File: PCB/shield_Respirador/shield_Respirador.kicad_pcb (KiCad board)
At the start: 2 copper layers, 137.3 x 102 mm, 29 parts, among them P1 Digital, P10 CONN_01X01, P11 CONN_01X01, P12 CONN_01X01, P13 CONN_01X01, P2 Power, P3 Analog, P4 Analog, P5 PWM, P6 PWM, P7 Communication, P8 CONN_01X01, P9 CONN_01X01

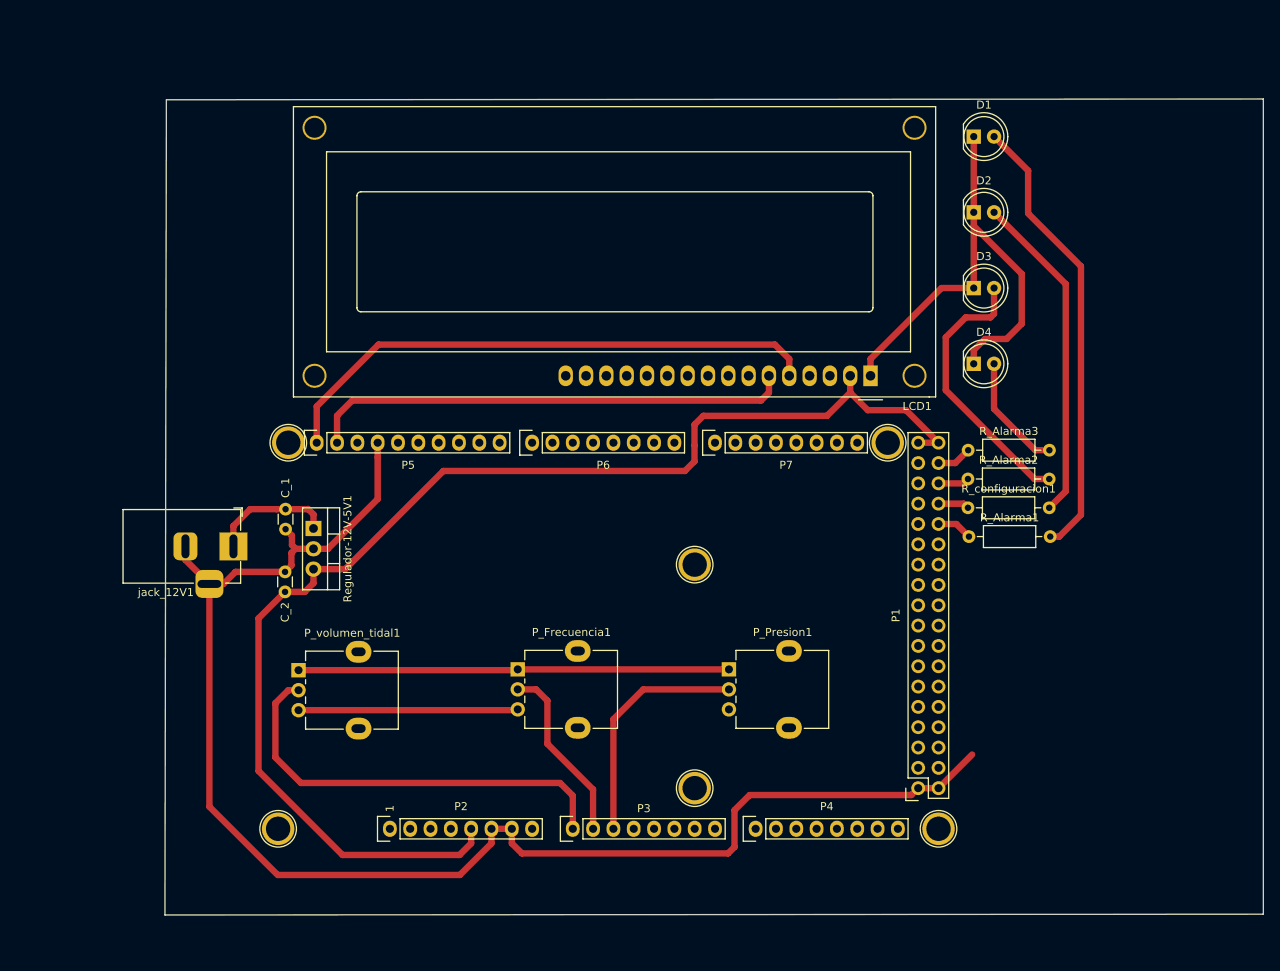
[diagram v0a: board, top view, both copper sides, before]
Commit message: version 0.4
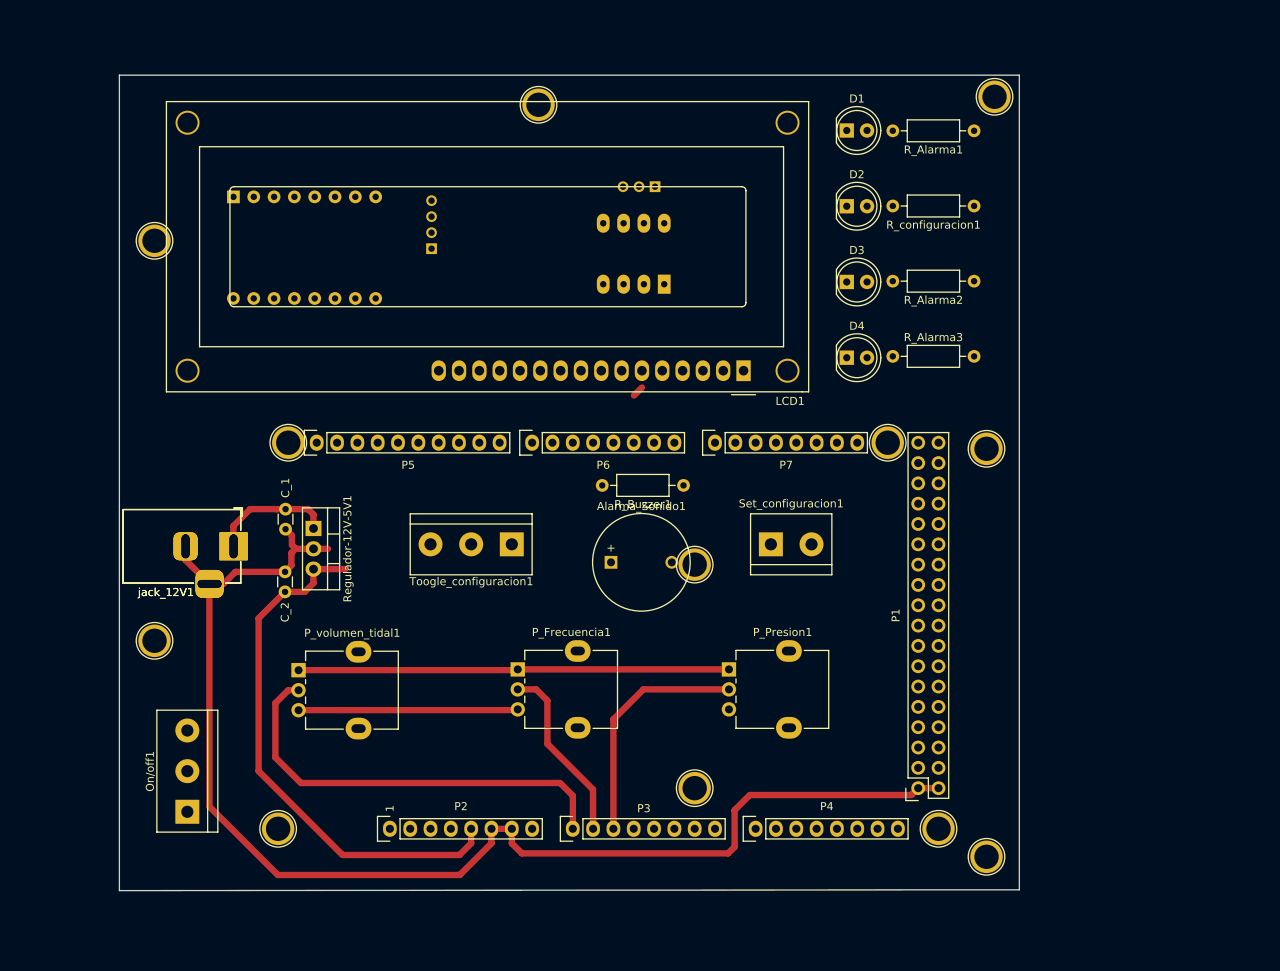
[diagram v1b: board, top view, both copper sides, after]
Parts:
- added Alarma_Sonido1: Buzzer, Buzzer_Beeper:MagneticBuzzer_ProSignal_ABI-009-RC, F.Cu at (159.0, 85.8)
- added Drivermotor1: Pololu_Breakout_DRV8825, Module:Pololu_Breakout-16_15.2x20.3mm, B.Cu at (111.8, 40.1)
- added Final_De_Carrera1: Conn_01x03_Female, Connector_PinSocket_2.00mm:PinSocket_1x03_P2.00mm_Vertical, B.Cu at (164.5, 38.9)
- added On/off1: SW_DPDT_x2, TerminalBlock:TerminalBlock_bornier-3_P5.08mm, F.Cu at (106.0, 117.0)
- added P10: CONN_01X01, Socket_Arduino_Mega:Arduino_1pin, F.Cu at (101.9, 95.6)
- added P10: CONN_01X01, Socket_Arduino_Mega:Arduino_1pin, F.Cu at (149.9, 28.6)
- added P10: CONN_01X01, Socket_Arduino_Mega:Arduino_1pin, F.Cu at (101.9, 45.6)
- added P10: CONN_01X01, Socket_Arduino_Mega:Arduino_1pin, F.Cu at (205.9, 71.6)
- added P10: CONN_01X01, Socket_Arduino_Mega:Arduino_1pin, F.Cu at (206.9, 27.6)
- added P10: CONN_01X01, Socket_Arduino_Mega:Arduino_1pin, F.Cu at (205.9, 122.6)
- added R_Buzzer1: 220, Resistor_THT:R_Axial_DIN0207_L6.3mm_D2.5mm_P10.16mm_Horizontal, F.Cu at (168.0, 76.2)
- added Sensor_Presion1: MPXA6115A, Package_DIP:DIP-8_W7.62mm_LongPads, B.Cu at (165.6, 51.1)
- added Set_configuracion1: SW_Push, TerminalBlock:TerminalBlock_bornier-2_P5.08mm, F.Cu at (178.9, 83.6)
- added Toogle_configuracion1: SW_Push_SPDT, TerminalBlock:TerminalBlock_bornier-3_P5.08mm, F.Cu at (146.6, 83.6)
- added conector_motor1: Conn_01x04_Female, Connector_PinSocket_2.00mm:PinSocket_1x04_P2.00mm_Vertical, B.Cu at (136.5, 46.6)
- added jack_12V1: Alimentacion_12V, Connector_BarrelJack:BarrelJack_Horizontal, F.Cu at (111.8, 83.8)
- moved R_Alarma1 50.7 mm to (204.3, 31.9), turned to 180 degrees
- moved R_configuracion1 37.7 mm to (204.3, 41.3), turned to 180 degrees
- moved R_Alarma2 24.7 mm to (204.3, 50.7), turned to 180 degrees
- moved D1 15.9 mm to (188.4, 31.8)
- moved D2 15.9 mm to (188.4, 41.3)
- moved D3 15.9 mm to (188.4, 50.8)
- moved D4 15.9 mm to (188.4, 60.2)
- moved LCD1 15.9 mm to (175.5, 61.9)
- moved R_Alarma3 15.0 mm to (194.2, 60.1)
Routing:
- net +5V: track 160.1 -> 66.8 mm
- net GND: track 244.0 -> 160.8 mm
- net /SCL: track 69.7 -> 0.00 mm
- net /SDA: track 60.7 -> 1.41 mm
- net Net-(D1-Pad2): track 56.8 -> 0.00 mm
- net Net-(D2-Pad2): track 41.5 -> 0.00 mm
- net Net-(D3-Pad2): track 34.6 -> 0.00 mm
- net Net-(D4-Pad2): track 14.7 -> 0.00 mm
- net /29: track 4.45 -> 0.00 mm
- net /23: track 4.37 -> 0.00 mm
- net /25: track 3.90 -> 0.00 mm
- net /27: track 3.89 -> 0.00 mm
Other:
- board size 137.3 x 102 mm -> 112.5 x 101.9 mm

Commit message: version 0.5 se termina esquematico y renderizacion
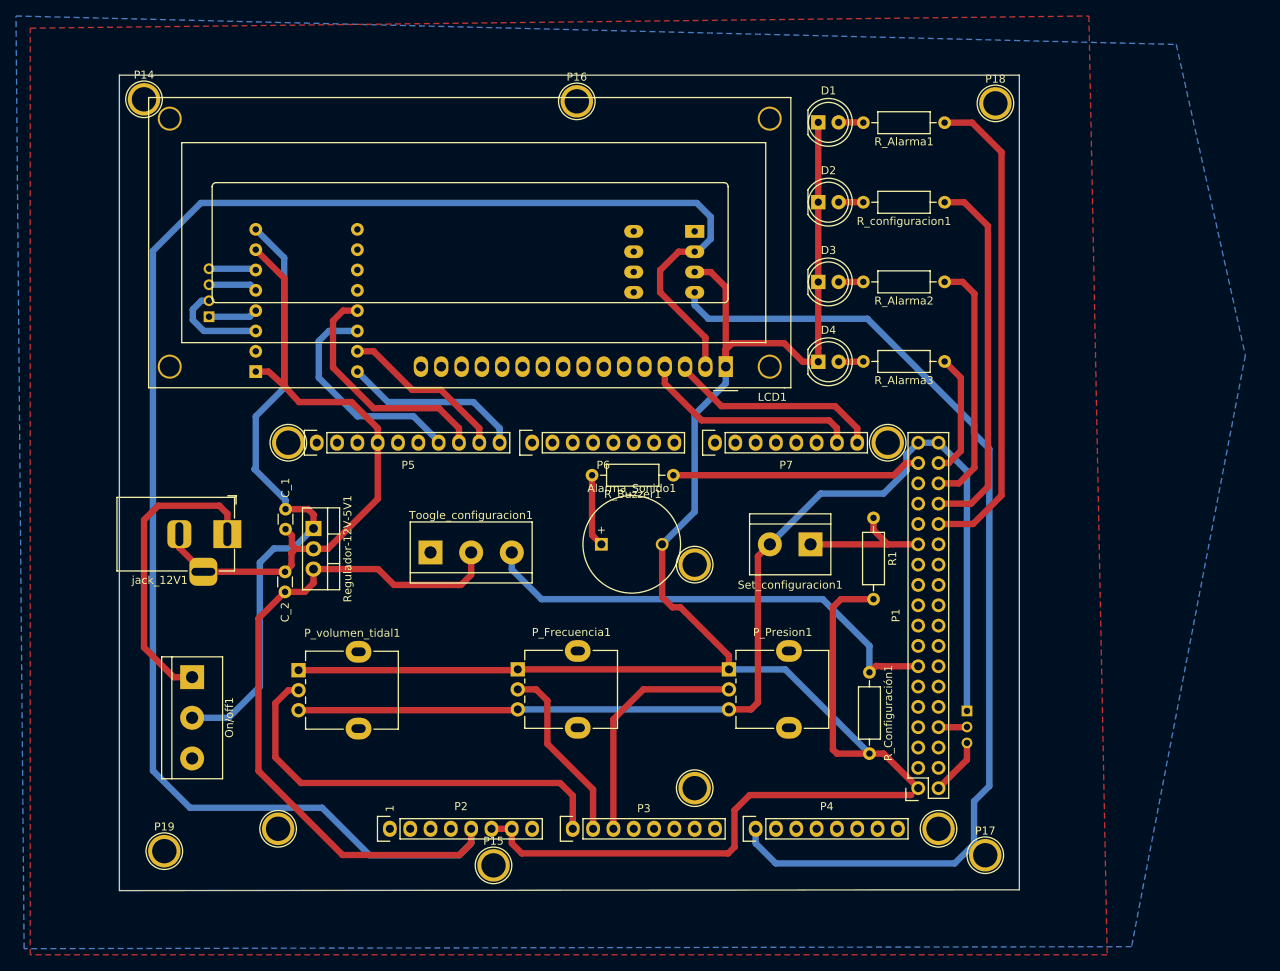
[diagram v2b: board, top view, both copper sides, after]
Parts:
- removed the P10 at (101.9, 95.6)
- removed the P10 at (149.9, 28.6)
- removed the P10 at (101.9, 45.6)
- removed the P10 at (205.9, 71.6)
- removed the P10 at (206.9, 27.6)
- removed the P10 at (205.9, 122.6)
- removed the jack_12V1 at (111.8, 83.8) (x2)
- added P14: CONN_01X01, Socket_Arduino_Mega:Arduino_1pin, F.Cu at (100.6, 27.9)
- added P15: CONN_01X01, Socket_Arduino_Mega:Arduino_1pin, F.Cu at (144.3, 123.7)
- added P16: CONN_01X01, Socket_Arduino_Mega:Arduino_1pin, F.Cu at (154.7, 28.2)
- added P17: CONN_01X01, Socket_Arduino_Mega:Arduino_1pin, F.Cu at (205.7, 122.4)
- added P18: CONN_01X01, Socket_Arduino_Mega:Arduino_1pin, F.Cu at (207.0, 28.4)
- added P19: CONN_01X01, Socket_Arduino_Mega:Arduino_1pin, F.Cu at (103.1, 121.9)
- added R1: R, Resistor_THT:R_Axial_DIN0207_L6.3mm_D2.5mm_P10.16mm_Horizontal, F.Cu at (191.8, 80.3)
- added R_Configuración1: 220, Resistor_THT:R_Axial_DIN0207_L6.3mm_D2.5mm_P10.16mm_Horizontal, F.Cu at (191.3, 99.6)
- added jack_12V1: Alimentacion_12V, Connector_BarrelJack:BarrelJack_Horizontal, F.Cu at (111.0, 82.3)
- Drivermotor1: value Pololu_Breakout_DRV8825 -> DRV8825
- moved Final_De_Carrera1 76.3 mm to (203.5, 104.4), turned to 180 degrees
- moved conector_motor1 29.1 mm to (108.7, 55.1)
- moved Drivermotor1 22.0 mm to (114.6, 62.0), turned to 0 degrees
- moved On/off1 16.8 mm to (106.6, 100.2), turned to 270 degrees
- moved Toogle_configuracion1 10.2 mm to (136.4, 84.6), turned to 0 degrees
- moved Sensor_Presion1 7.62 mm to (169.4, 44.5), turned to 180 degrees
- moved R_Alarma3 6.51 mm to (200.7, 60.7), turned to 180 degrees
- moved Set_configuracion1 4.95 mm to (183.9, 83.6), turned to 180 degrees
- moved R_Alarma1 3.82 mm to (200.7, 30.9)
- moved R_configuracion1 3.71 mm to (200.7, 40.8)
- moved D1 3.70 mm to (184.9, 30.8)
- moved R_Alarma2 3.68 mm to (200.7, 50.8)
- moved D4 3.59 mm to (184.9, 60.7)
- moved D2 3.59 mm to (184.9, 40.8)
- moved D3 3.56 mm to (184.9, 50.8)
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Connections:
- Drivermotor1 pad 1: Net-(Drivermotor1-Pad1) -> GND
- Drivermotor1 pad 13: Net-(Drivermotor1-Pad13) -> /10(**)
- Drivermotor1 pad 14: Net-(Drivermotor1-Pad14) -> /11(**)
- Drivermotor1 pad 15: Net-(Drivermotor1-Pad15) -> /9(**)
- Drivermotor1 pad 16: Net-(Drivermotor1-Pad16) -> /8(**)
- Drivermotor1 pad 7: Net-(Drivermotor1-Pad7) -> GND
- Drivermotor1 pad 8: Net-(Drivermotor1-Pad8) -> +12V
- Final_De_Carrera1 pad 1: Net-(Final_De_Carrera1-Pad1) -> +5V
- Final_De_Carrera1 pad 2: Net-(Final_De_Carrera1-Pad2) -> /49
- Final_De_Carrera1 pad 3: Net-(Final_De_Carrera1-Pad3) -> GND
- LCD1 pad 3: Net-(LCD1-Pad3) -> /21(SCL)
- LCD1 pad 4: Net-(LCD1-Pad4) -> /20(SDA)
- LCD1 pad 5: /SCL -> Net-(LCD1-Pad5)
- LCD1 pad 6: /SDA -> Net-(LCD1-Pad6)
- P_Frecuencia1 pad 1: Net-(P_Frecuencia1-Pad1) -> GND
- P_Frecuencia1 pad 3: Net-(P_Frecuencia1-Pad3) -> +5V
- P_Presion1 pad 1: Net-(P_Frecuencia1-Pad1) -> GND
- P_Presion1 pad 3: Net-(P_Frecuencia1-Pad3) -> +5V
- P_volumen_tidal1 pad 1: Net-(P_Frecuencia1-Pad1) -> GND
- P_volumen_tidal1 pad 3: Net-(P_Frecuencia1-Pad3) -> +5V
- R_Buzzer1 pad 1: /31 -> /22
- Sensor_Presion1 pad 2: Net-(Sensor_Presion1-Pad2) -> +5V
- Sensor_Presion1 pad 3: Net-(Sensor_Presion1-Pad3) -> GND
- Sensor_Presion1 pad 4: Net-(Sensor_Presion1-Pad4) -> /A8
- Set_configuracion1 pad 1: Net-(Set_configuracion1-Pad1) -> /30
- Set_configuracion1 pad 2: Net-(Set_configuracion1-Pad2) -> +5V
- Toogle_configuracion1 pad 2: Net-(Toogle_configuracion1-Pad2) -> +5V
- Toogle_configuracion1 pad 3: Net-(Toogle_configuracion1-Pad3) -> /42
- conector_motor1 pad 1: Net-(conector_motor1-Pad1) -> Net-(Drivermotor1-Pad4)
- conector_motor1 pad 2: Net-(conector_motor1-Pad2) -> Net-(Drivermotor1-Pad3)
- conector_motor1 pad 3: Net-(conector_motor1-Pad3) -> Net-(Drivermotor1-Pad5)
- conector_motor1 pad 4: Net-(conector_motor1-Pad4) -> Net-(Drivermotor1-Pad6)
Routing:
- net +5V: track 66.8 -> 437.0 mm
- net GND: track 160.8 -> 366.7 mm
- net /A8: track 0.00 -> 127.8 mm
- net +12V: track 15.5 -> 79.2 mm
- net /29: track 0.00 -> 60.9 mm
- net /42: track 0.00 -> 60.6 mm
- net Net-(P_Frecuencia1-Pad1): track 53.8 -> 0.00 mm
- net /27: track 0.00 -> 46.3 mm
- net Net-(On/off1-Pad1): track 0.00 -> 37.6 mm
- net /25: track 0.00 -> 31.4 mm
- net /22: track 0.00 -> 31.2 mm
- net /10(**): track 0.00 -> 30.1 mm
- net /11(**): track 0.00 -> 28.4 mm
- net /20(SDA): track 0.00 -> 27.8 mm
- net Net-(P_Frecuencia1-Pad3): track 27.4 -> 0.00 mm
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- added copper zone on B.Cu, net (none)
- added copper zone on F.Cu, net (none)
